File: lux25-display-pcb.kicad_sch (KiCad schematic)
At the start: 0 parts

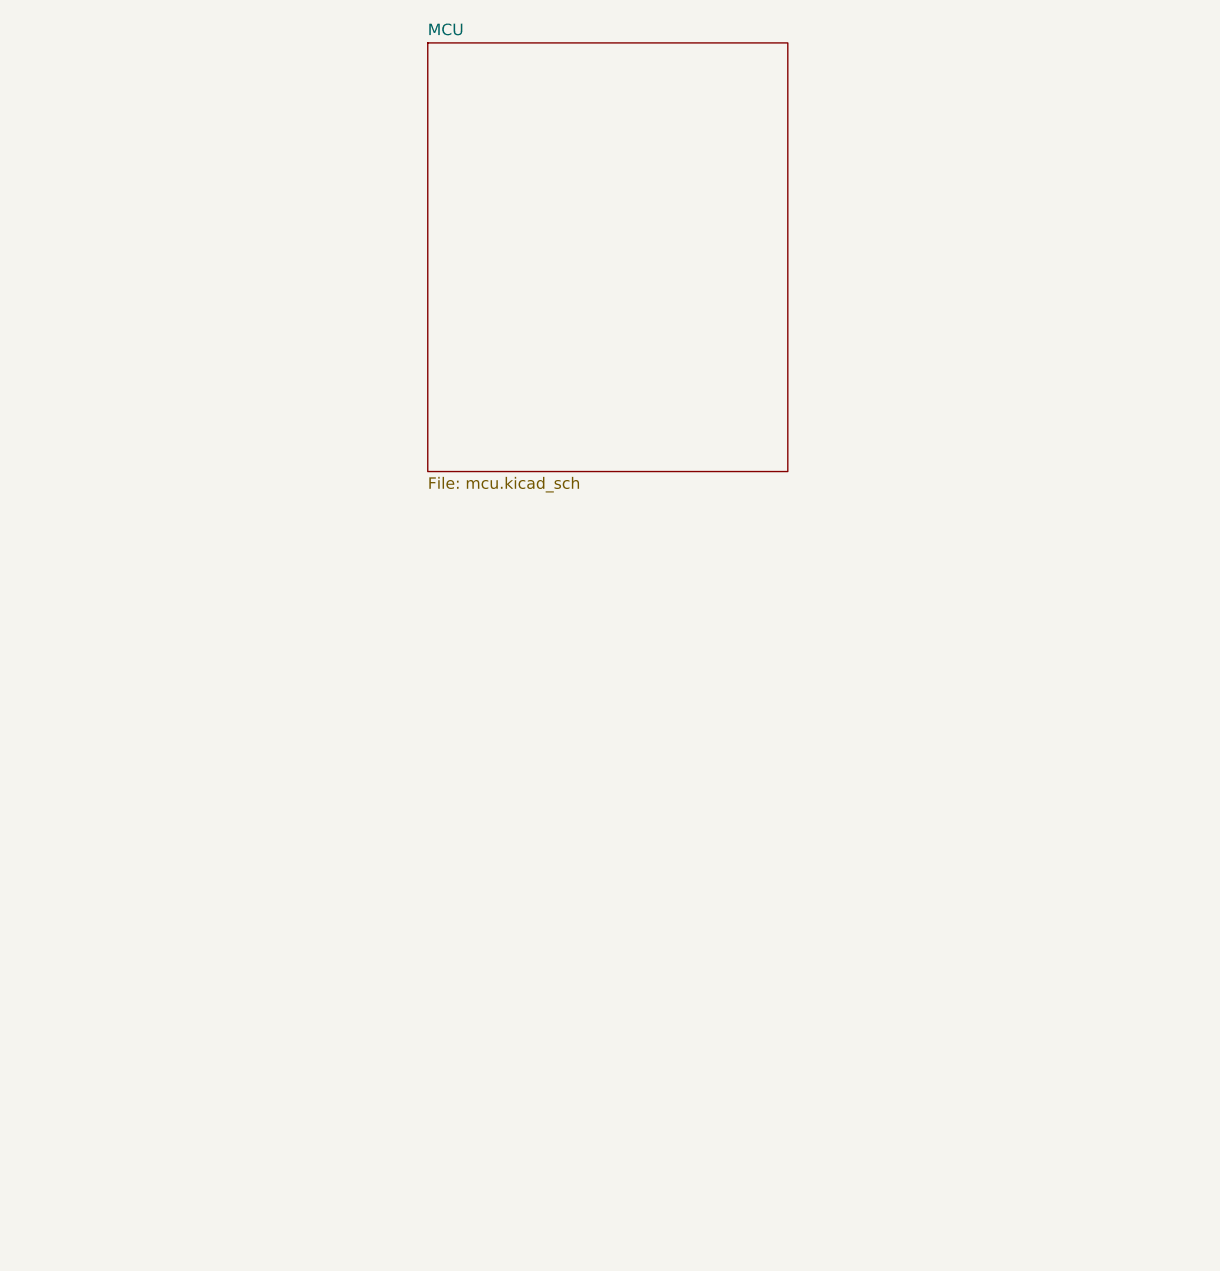
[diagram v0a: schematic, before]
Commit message: Finished Layout
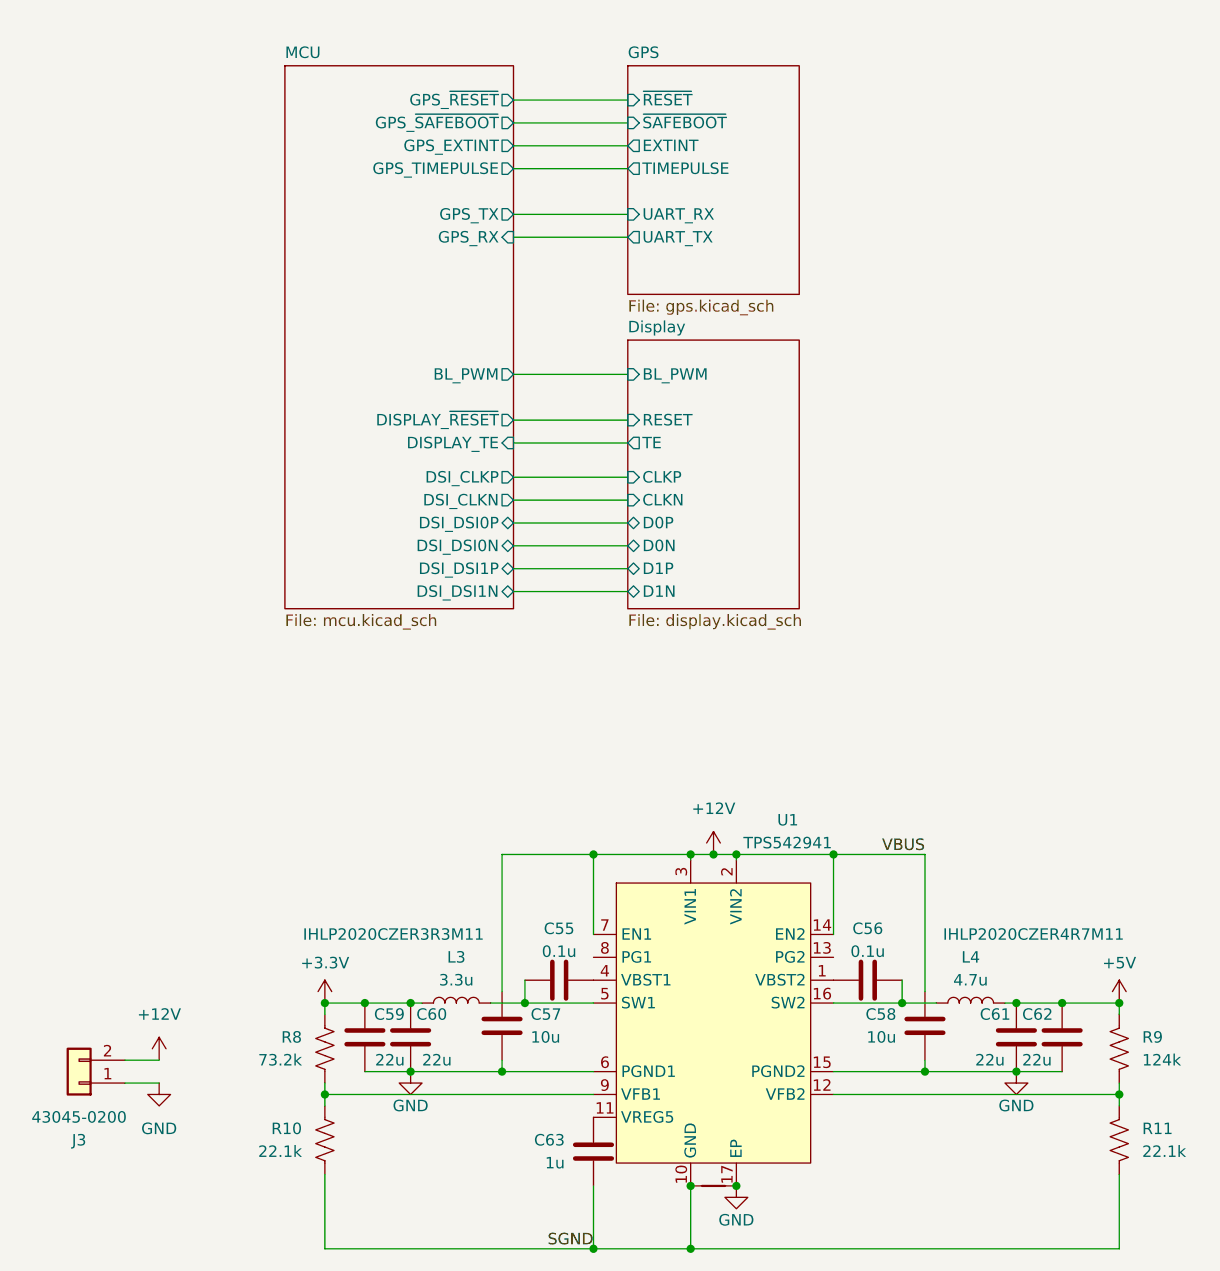
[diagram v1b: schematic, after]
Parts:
- added C55, C56: 0.1u, Capacitor_SMD:C_0402_1005Metric, symbol Device:C
- added C57, C58: 10u, Capacitor_SMD:C_0603_1608Metric, symbol Device:C
- added C59, C60, C61, C62: 22u, Capacitor_SMD:C_0805_2012Metric, symbol Device:C
- added C63: 1u, Capacitor_SMD:C_0402_1005Metric, symbol Device:C
- added J3: 43045-0200, Molex_Custom:Molex_Micro-Fit_3.0_43045-0200_2x01_P3.00mm_Horizontal, symbol Connector_Generic:Conn_01x02
- added L3: 3.3u, Inductor_SMD:L_Vishay_IHLP-2020, symbol Device:L
- added L4: 4.7u, Inductor_SMD:L_Vishay_IHLP-2020, symbol Device:L
- added NT2: NetTie_2, NetTies:NetTie_2_0.25mm, symbol Device:NetTie_2
- added R10, R11: 22.1k, Resistor_SMD:R_0402_1005Metric, symbol Device:R_US
- added R8: 73.2k, Resistor_SMD:R_0402_1005Metric, symbol Device:R_US
- added R9: 124k, Resistor_SMD:R_0402_1005Metric, symbol Device:R_US
- added U1: TPS542941, Package_DFN_QFN:Texas_RSA_VQFN-16-1EP_4x4mm_P0.65mm_EP2.7x2.7mm_ThermalVias, symbol TexasInstruments:TPS542941RSA
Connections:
- new net: C63.2, U1.11 (VREG5)
- new net: R11.1, R9.2, U1.12 (VFB2)
- new net: C56.2, L4.1, U1.16 (SW2)
- new net: C56.1, U1.1 (VBST2)
- new net: R10.1, R8.2, U1.9 (VFB1)
- new net: C55.1, L3.1, U1.5 (SW1)
- new net: C55.2, U1.4 (VBST1)
- new net +12V: C57.2, C58.2, J3.2 (Pin_2), U1.14 (EN2), U1.2 (VIN2), U1.3 (VIN1), U1.7 (EN1)
- new net +3.3V: C59.2, C60.2, L3.2, R8.1
- new net +5V: C61.2, C62.2, L4.2, R9.1
- new net GND: C57.1, C58.1, C59.1, C60.1, C61.1, C62.1, J3.1 (Pin_1), NT2.2, U1.15 (PGND2), U1.17 (EP), U1.6 (PGND1)
- new net SGND: C63.1, NT2.1, R10.2, R11.2, U1.10 (GND)
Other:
- added sheet Display (display.kicad_sch)
- added sheet GPS (gps.kicad_sch)
- sheet MCU ports: added BL_PWM, DISPLAY_TE, DISPLAY_~{RESET}, DSI_CLKN, DSI_CLKP, DSI_DSI0N, DSI_DSI0P, DSI_DSI1N, DSI_DSI1P, GPS_EXTINT, GPS_RX, GPS_TIMEPULSE, GPS_TX, GPS_~{RESET}, GPS_~{SAFEBOOT}; removed none
